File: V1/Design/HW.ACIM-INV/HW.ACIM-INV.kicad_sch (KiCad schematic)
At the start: 7 parts

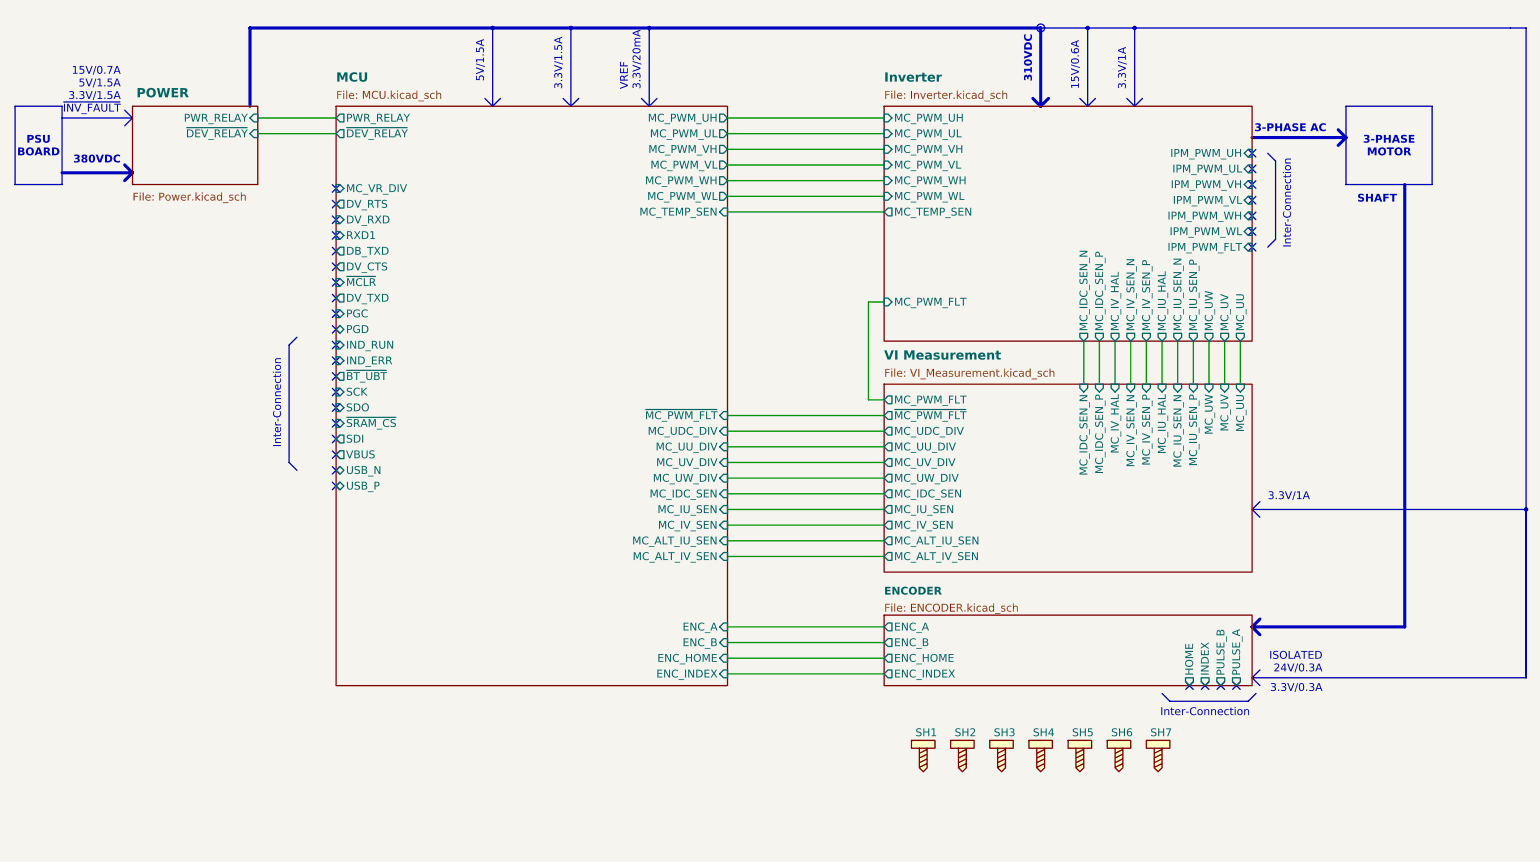
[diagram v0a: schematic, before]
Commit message: V1 schematic update 9
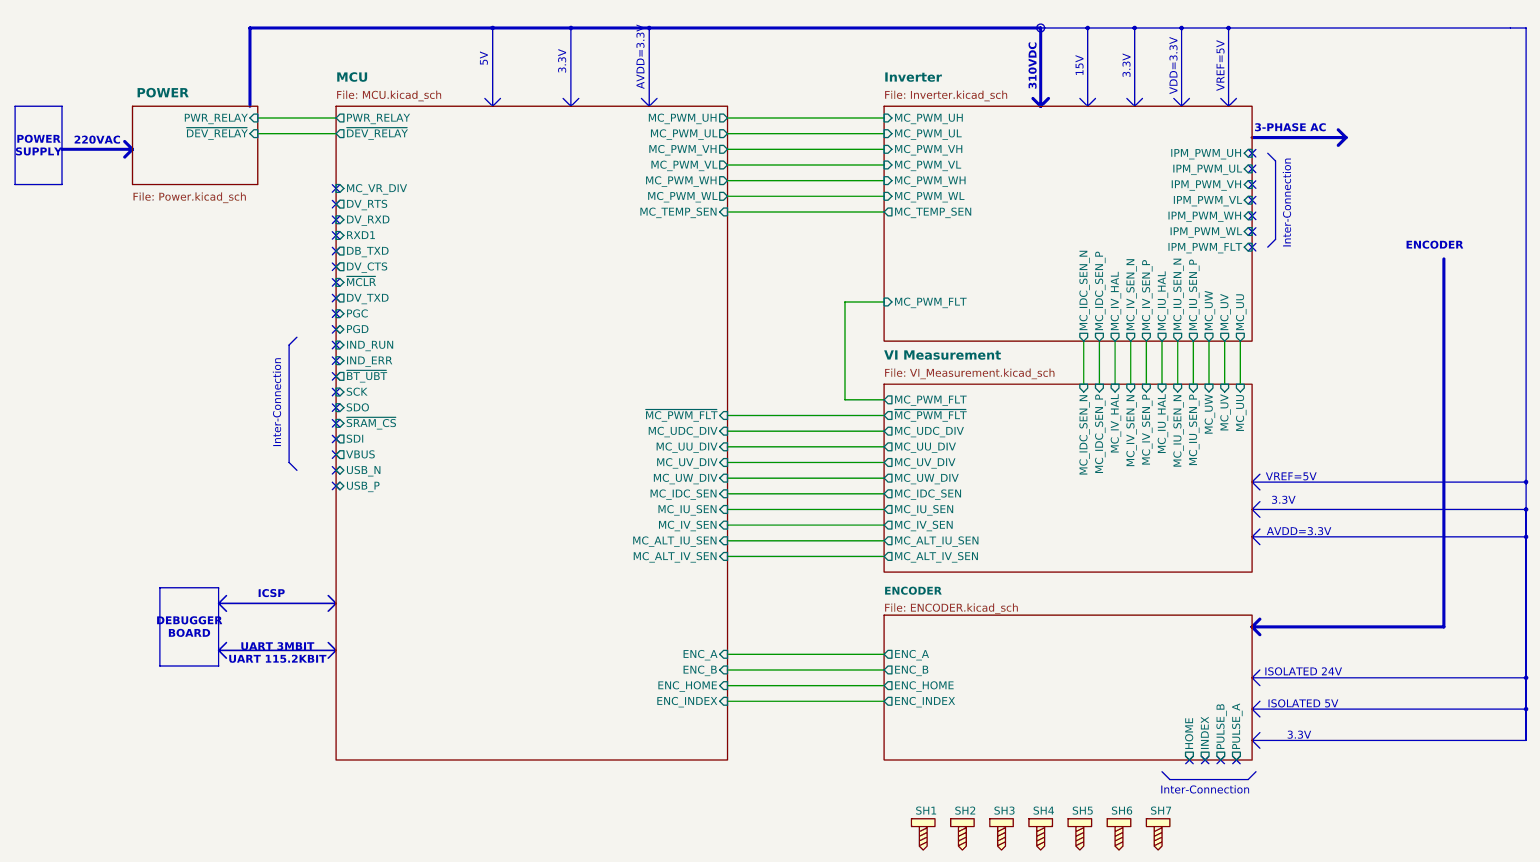
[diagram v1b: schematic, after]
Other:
- note added: "15V"
- note added: "220VAC"
- note added: "3.3V"
- note added: "5V"
- note added: "AVDD=3.3V"
- note added: "ENCODER"
- note added: "ICSP"
- note added: "ISOLATED 24V"
- note added: "ISOLATED 5V"
- note added: "UART 3MBIT UART 115.2KBIT"
- note added: "VDD=3.3V"
- note added: "VREF=5V"
- note removed: "15V/0.6A"
- note removed: "15V/0.7A 5V/1.5A 3.3V/1.5A ~{INV_FAULT}"
- note removed: "3.3V/0.3A"
- note removed: "3.3V/1.5A"
- note removed: "3.3V/1A"
- note removed: "380VDC"
- note removed: "5V/1.5A"
- note removed: "ISOLATED 24V/0.3A"
- note removed: "SHAFT"
- note removed: "VREF 3.3V/20mA"
- moved on the sheet: SH1, SH2, SH3, SH4, SH5, SH6, SH7
